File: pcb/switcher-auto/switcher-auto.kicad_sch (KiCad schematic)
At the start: 27 parts, among them J0 MD-90SM, J5 Conn_02x22_Top_Bottom, SW1 SW_Push, SW2 SW_Push, U1 CD74HC4067SM96, U2 CD74HC4067SM96, U3 CD74HC4067SM96, U4 CD74HC4067SM96, U5 CD74HC4067SM96, U6 CD74HC4067SM96, U7 CD74HC4067SM96

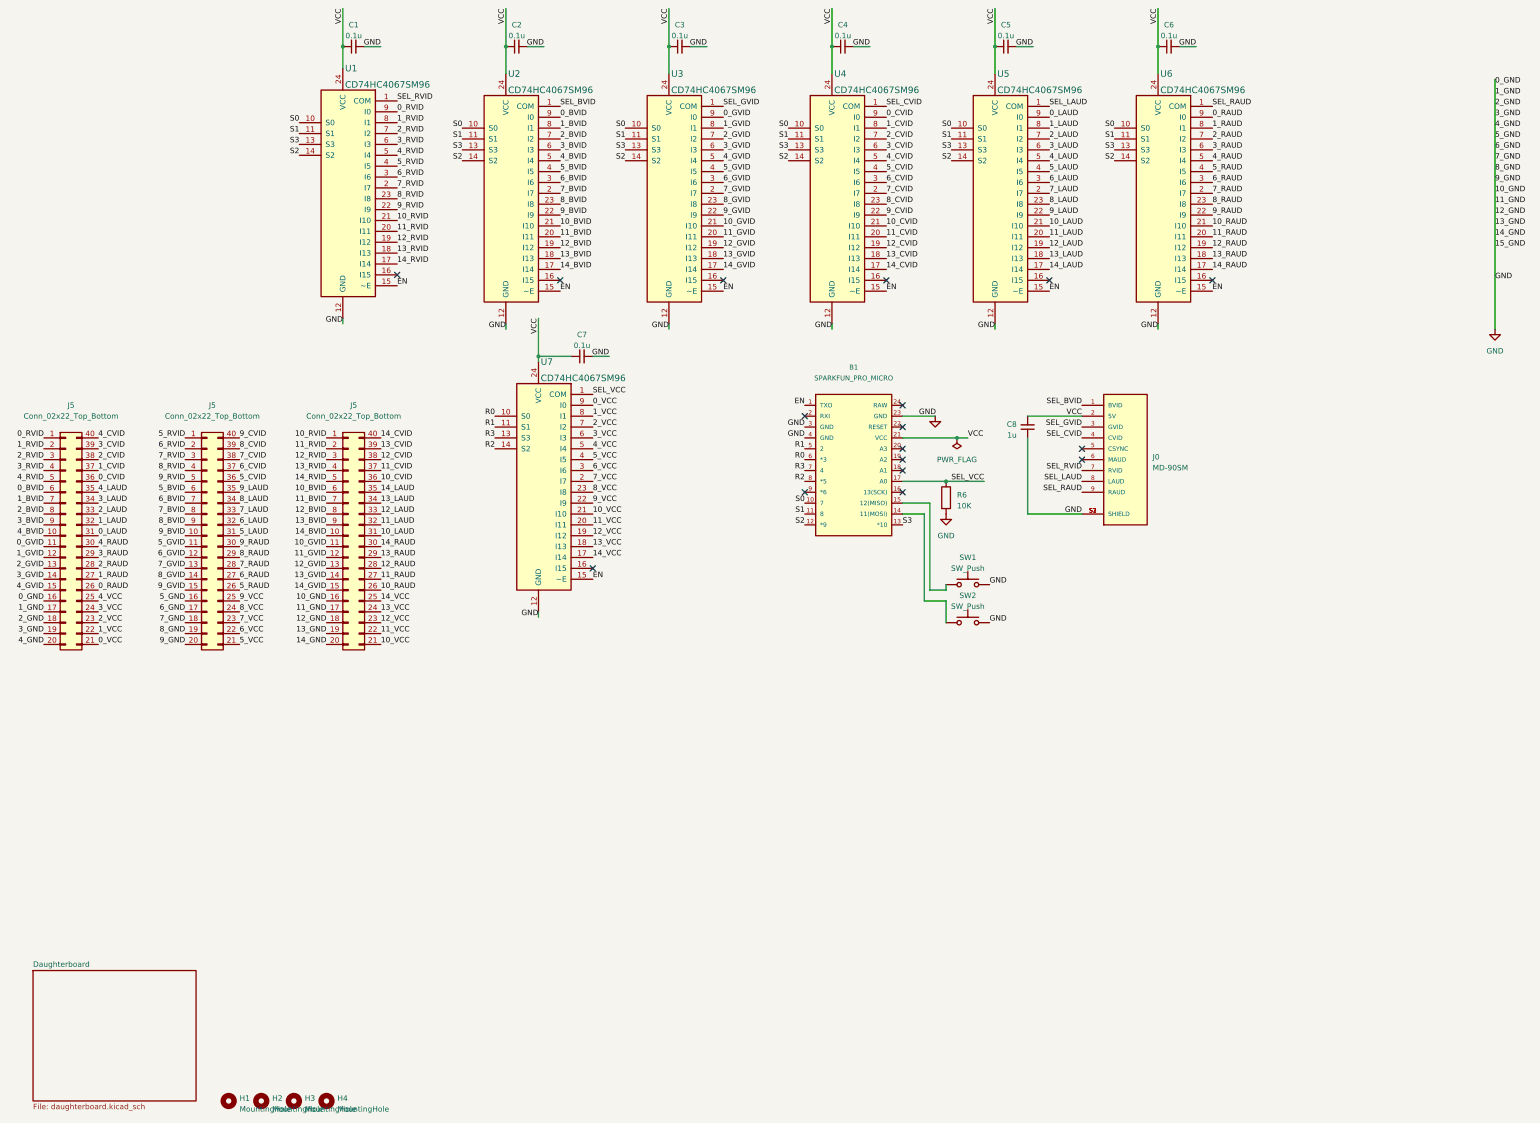
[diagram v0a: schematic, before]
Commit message: WIP
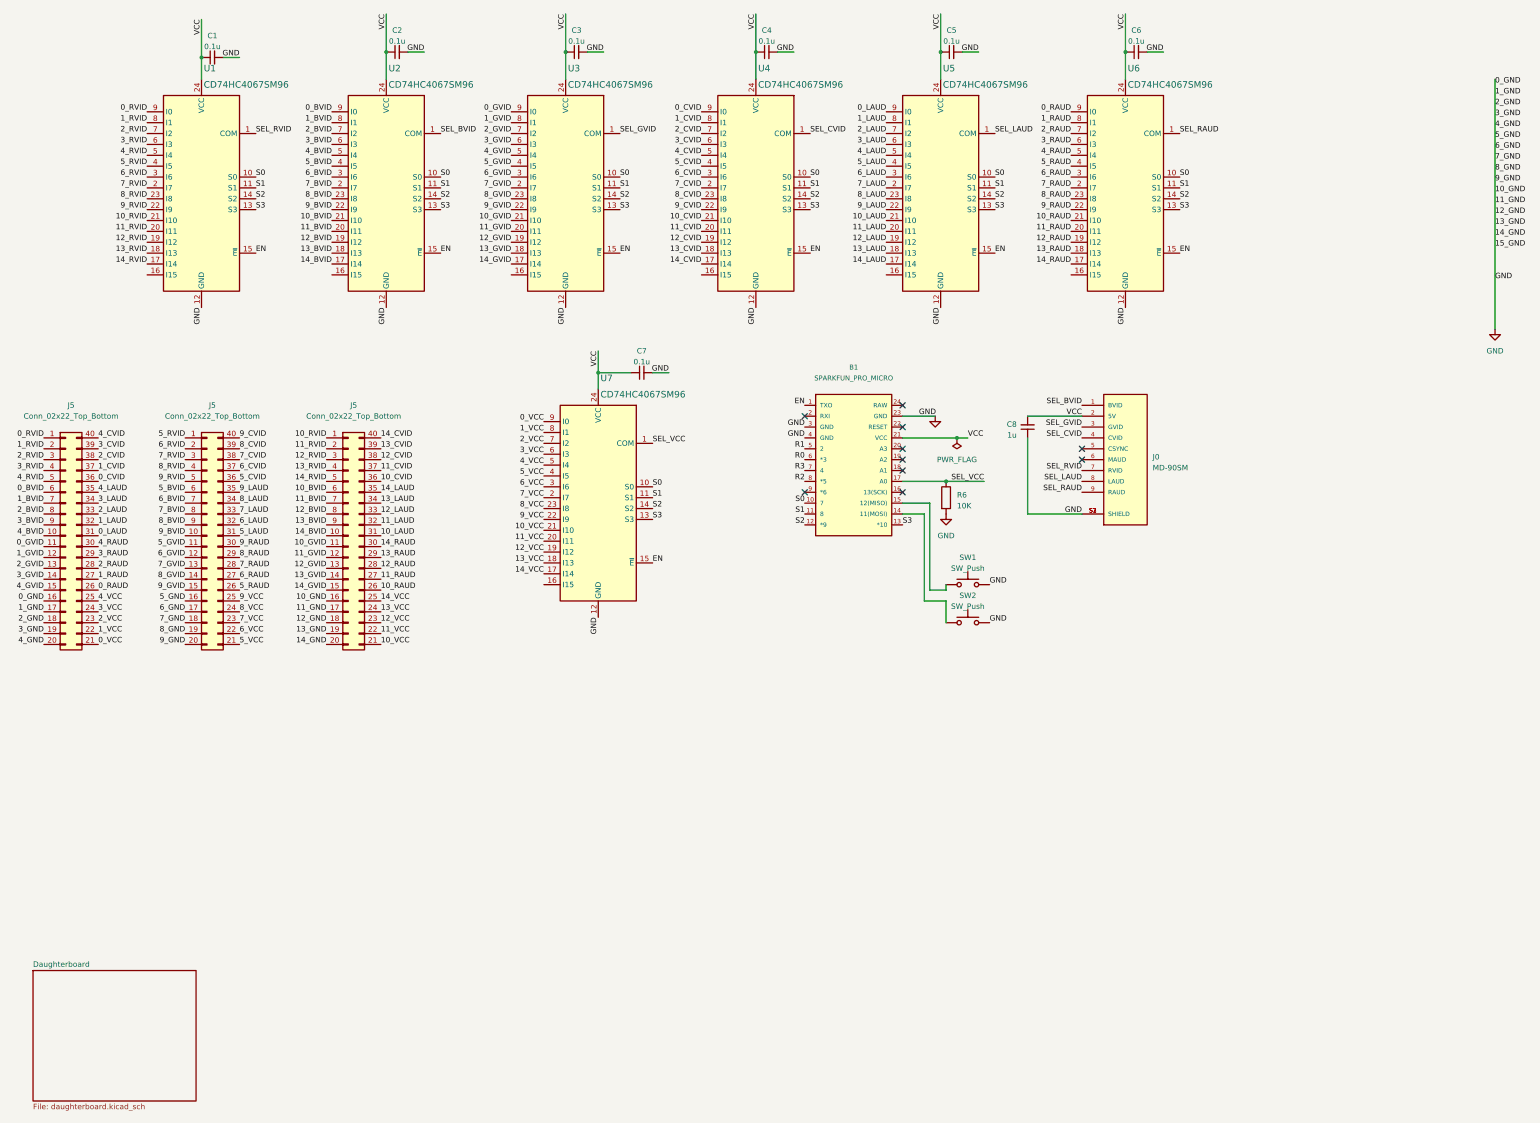
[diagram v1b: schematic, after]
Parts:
- removed H1, H2, H3, H4: MountingHole, MountingHole:MountingHole_2.5mm, symbol Mechanical:MountingHole
- U1, U2, U3, U4, U5, U6, U7: footprint Package_SO:SSOP-24_5.3x8.2mm_P0.65mm -> Package_SO:SOIC-24W_7.5x15.4mm_P1.27mm; symbol dk_Interface-Analog-Switches-Multiplexers-Demultiplexers:CD74HC4067SM96 -> REB-DIN:CD4067BM96
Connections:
- net R0: no longer U7.10 (S0)
- net R1: no longer U7.11 (S1)
- net R2: no longer U7.14 (S2)
- net R3: no longer U7.13 (S3)
- net S0: now also U7.10 (S0)
- net S1: now also U7.11 (S1)
- net S2: now also U7.14 (S2)
- net S3: now also U7.13 (S3)
- no-connect marks 17 -> 10
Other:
- moved on the sheet: C1, C2, C3, C4, C5, C6, C7, U1, U2, U3, U4, U5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
